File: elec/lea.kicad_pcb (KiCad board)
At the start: 2 copper layers, 53.3 x 71.1 mm, 16 parts, among them J1 Servomoteur, J2 Jack, J3 Screw_Terminal_01x02, SW1 SW_SPDT

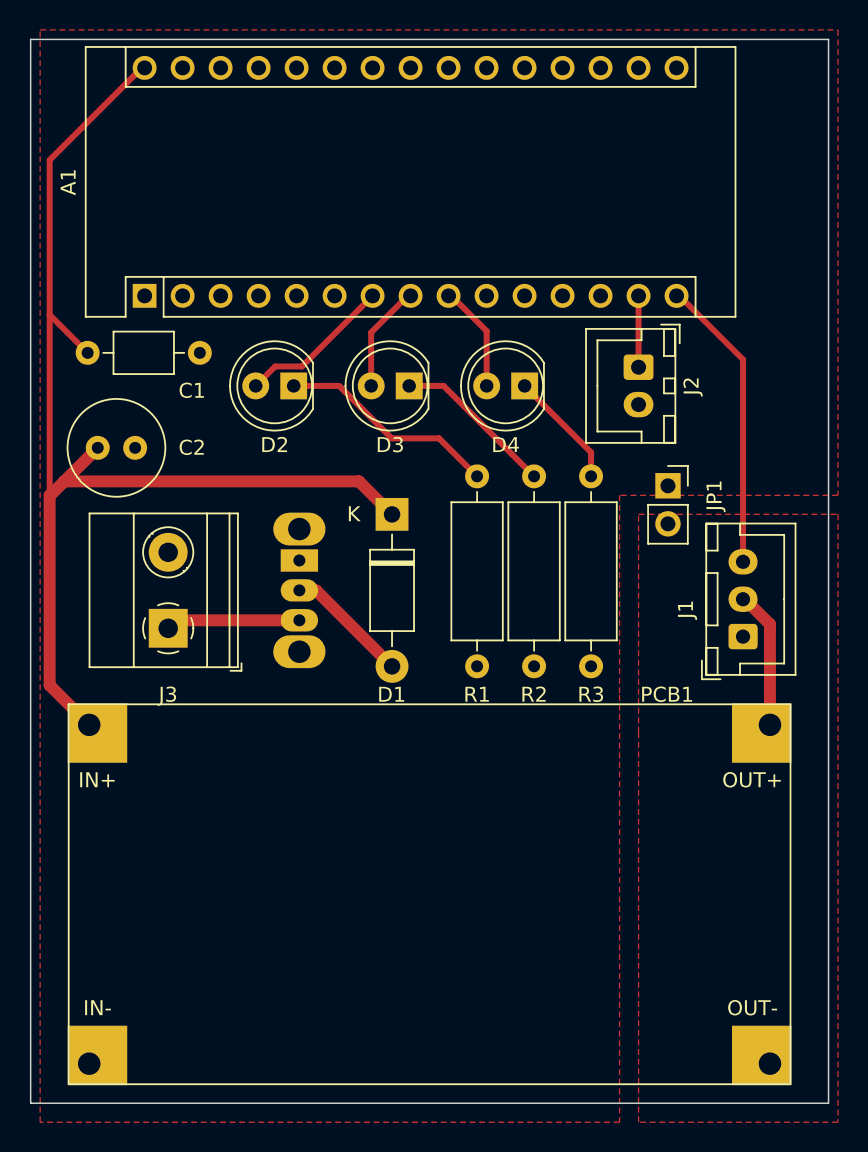
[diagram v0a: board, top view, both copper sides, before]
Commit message: version du pcb usinable au fablab
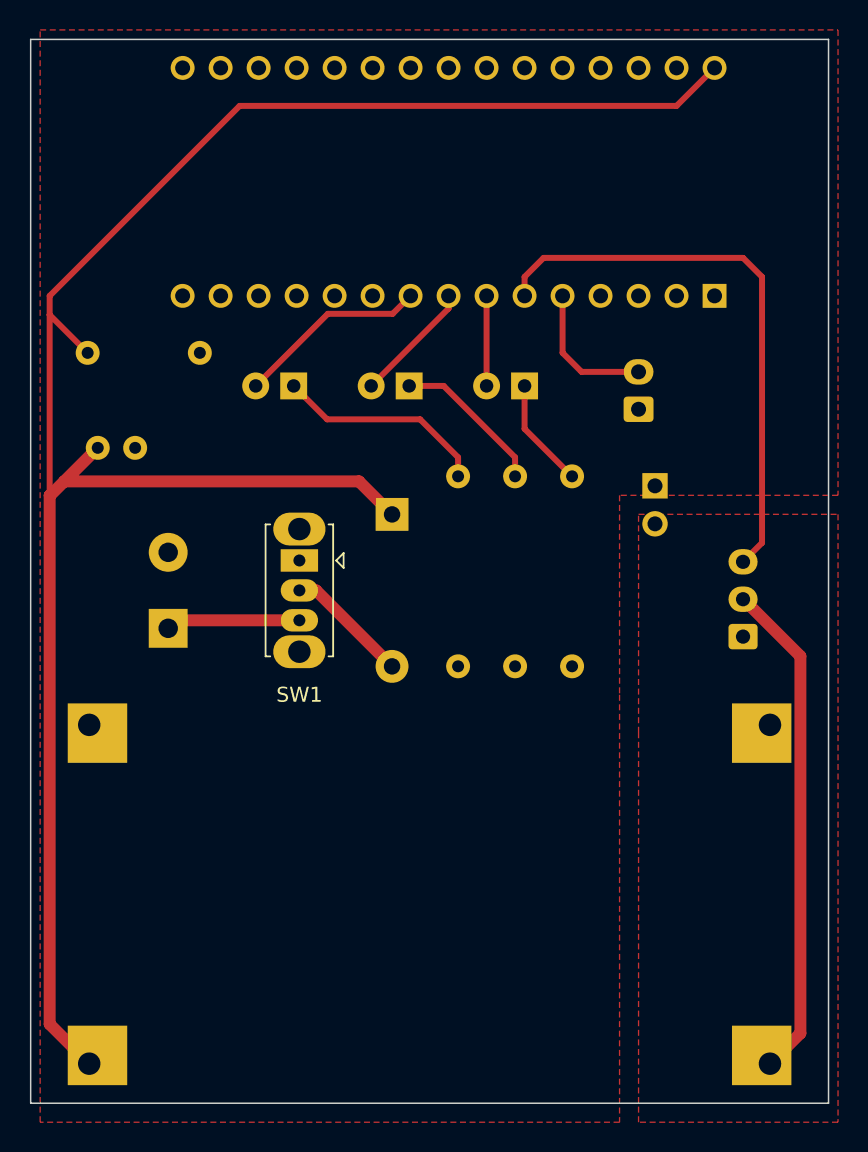
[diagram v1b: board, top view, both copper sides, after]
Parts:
- A1, C1, C2, D1, D2, D3, D4, J1, J2, J3, JP1, PCB1, R1, R2, R3: moved to B.Cu
- SW1: moved to F.Cu
- moved A1 38.1 mm to (222.2, 74.3)
- moved D4 15.4 mm to (194.1, 80.3)
- moved D2 15.4 mm to (209.6, 80.3)
- moved R3 8.89 mm to (205.1, 99.1)
- moved R1 6.35 mm to (212.7, 99.1)
- moved J2 2.81 mm to (217.2, 81.9), turned to 90 degrees
- moved R2 1.27 mm to (208.9, 99.1)
- moved JP1 0.86 mm to (218.3, 87.0), turned to 180 degrees
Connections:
- A1 pad 14: /JCK -> unconnected-(A1-Pad14)
- A1 pad 15: /PWM -> unconnected-(A1-Pad15)
- A1 pad 5: unconnected-(A1-Pad5) -> /JCK
- A1 pad 6: unconnected-(A1-Pad6) -> /PWM
- J2 pad 1: /JCK -> GND
- J2 pad 2: GND -> /JCK
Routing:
- net /VIN: track 78.8 -> 134.1 mm
- net /V1: track 9.22 -> 33.5 mm
- net /PWM: track 19.8 -> 37.8 mm
- net Net-(D2-Pad1): track 14.8 -> 7.36 mm
- net Net-(D4-Pad1): track 7.88 -> 14.2 mm
- net /D6: track 7.26 -> 12.8 mm
- net /JCK: track 4.96 -> 9.42 mm
- net /D4: track 10.3 -> 6.02 mm
- net /D5: track 7.30 -> 8.16 mm
- net Net-(D3-Pad1): track 10.9 -> 10.3 mm
